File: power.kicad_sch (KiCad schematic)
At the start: 32 parts, among them U101 xc7z010clg400, U401 TPS621351, U402 TLV62130RGTT, U403 TLV62130RGTT, U404 SPX3819M5-L-3-3

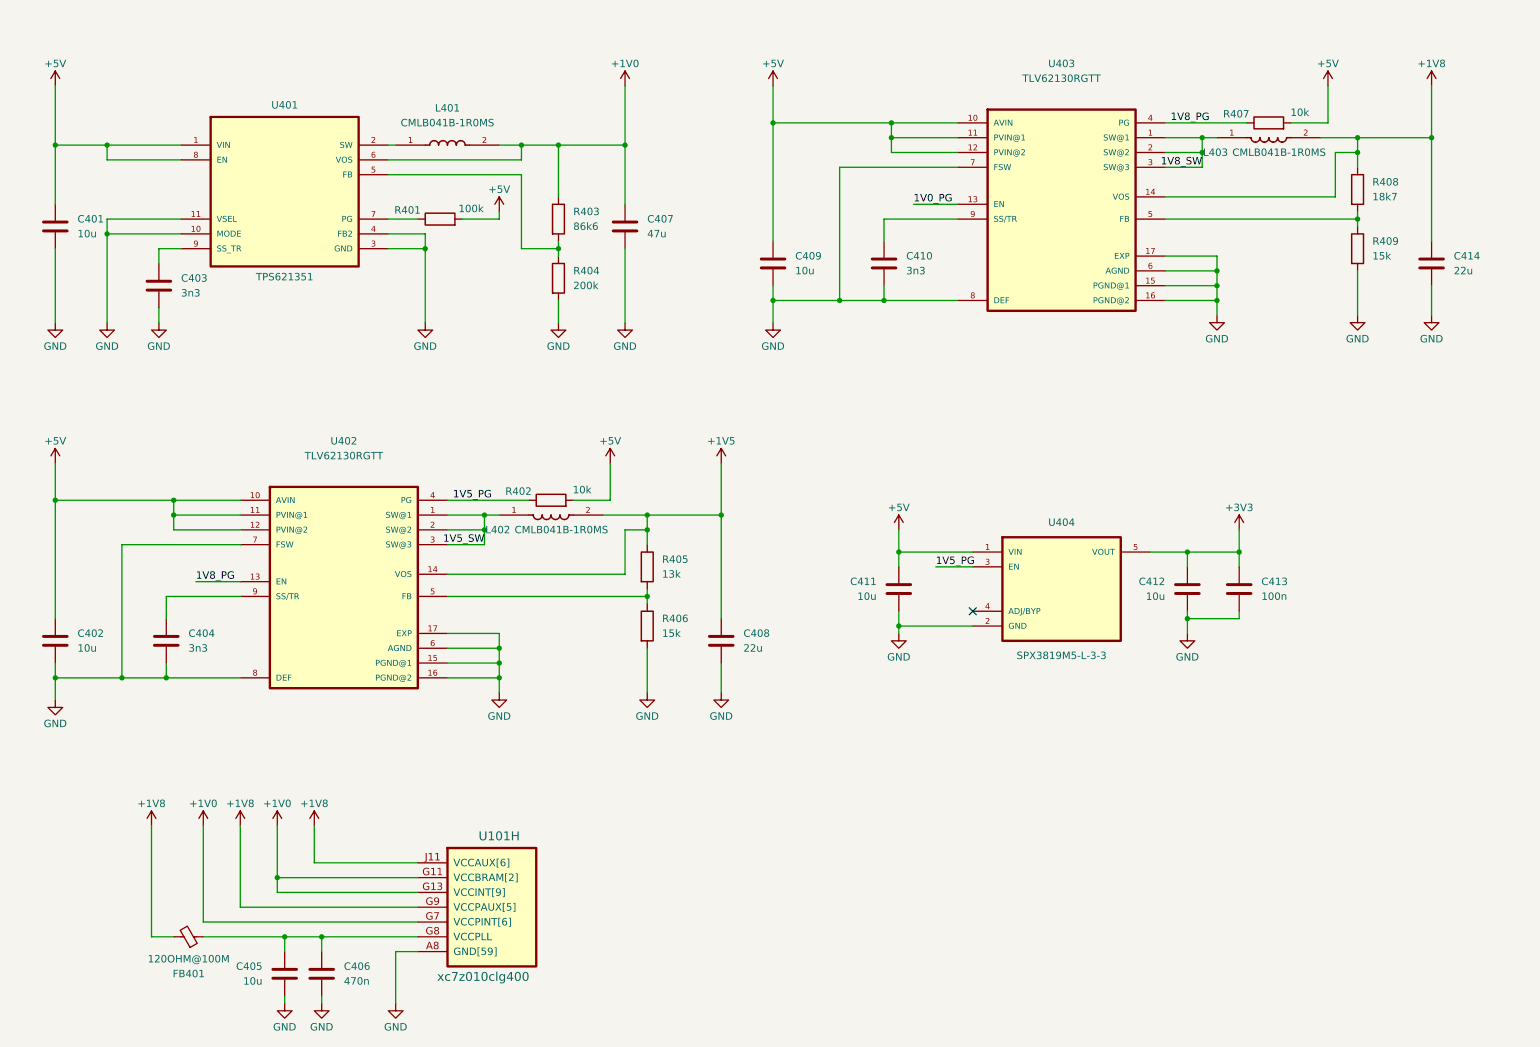
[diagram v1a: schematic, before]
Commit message: feat: continue sch design
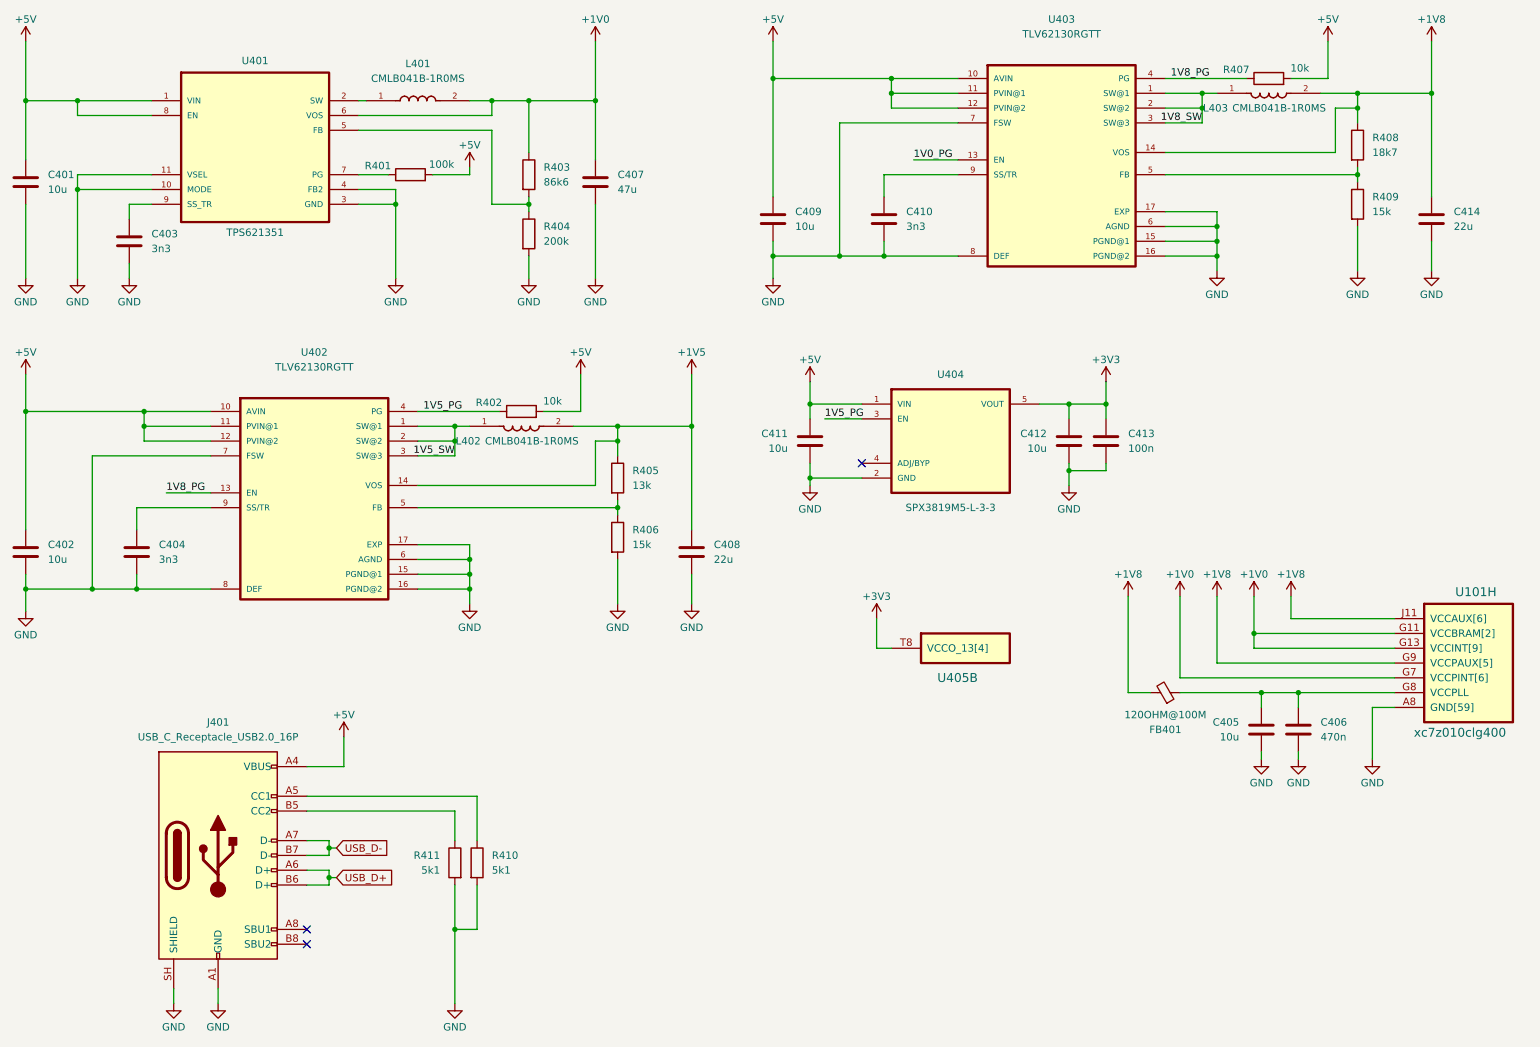
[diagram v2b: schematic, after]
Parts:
- added J401: USB_C_Receptacle_USB2.0_16P, symbol Connector:USB_C_Receptacle_USB2.0_16P
- added R410, R411: 5k1, symbol Device:R
- added U405: xc7z010clg400, Package_BGA:Xilinx_CLG400, symbol Xilinx7:xc7z010clg400
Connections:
- net +3V3: now also U405.T8 (VCCO_13[4]), U405.U11 (VCCO_13[4]), U405.W7 (VCCO_13[4]), U405.Y10 (VCCO_13[4])
- net +5V: now also J401.A4 (VBUS), J401.A9 (VBUS), J401.B4 (VBUS), J401.B9 (VBUS)
- net GND: now also J401.A1 (GND), J401.A12 (GND), J401.B1 (GND), J401.B12 (GND), J401.SH (SHIELD), R410.2, R411.2
- new net: J401.A5 (CC1), R410.1
- new net: J401.B5 (CC2), R411.1
- new net USB_D+: J401.A6 (D+), J401.B6 (D+)
- new net USB_D-: J401.A7 (D-), J401.B7 (D-)
- no-connect marks 1 -> 3
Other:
- moved on the sheet: C401, C402, C403, C404, C405, C406, C407, C408, C409, C410, C411, C412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
